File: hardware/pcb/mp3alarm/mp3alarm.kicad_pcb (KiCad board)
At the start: 2 copper layers, 67 x 54 mm, 30 parts, among them IC1 RDA5807FP, J0 debug, J1 AUDIO, J10 Conn_Coaxial, J2 SW0, J3 SW1, J4 SW2, J5 I2C, J6 TM1637, J7 microSD, J8 5V, J9 ANT, U1 UDA1334A_Breakout, U2 mini_esp32, Y1 Crystal

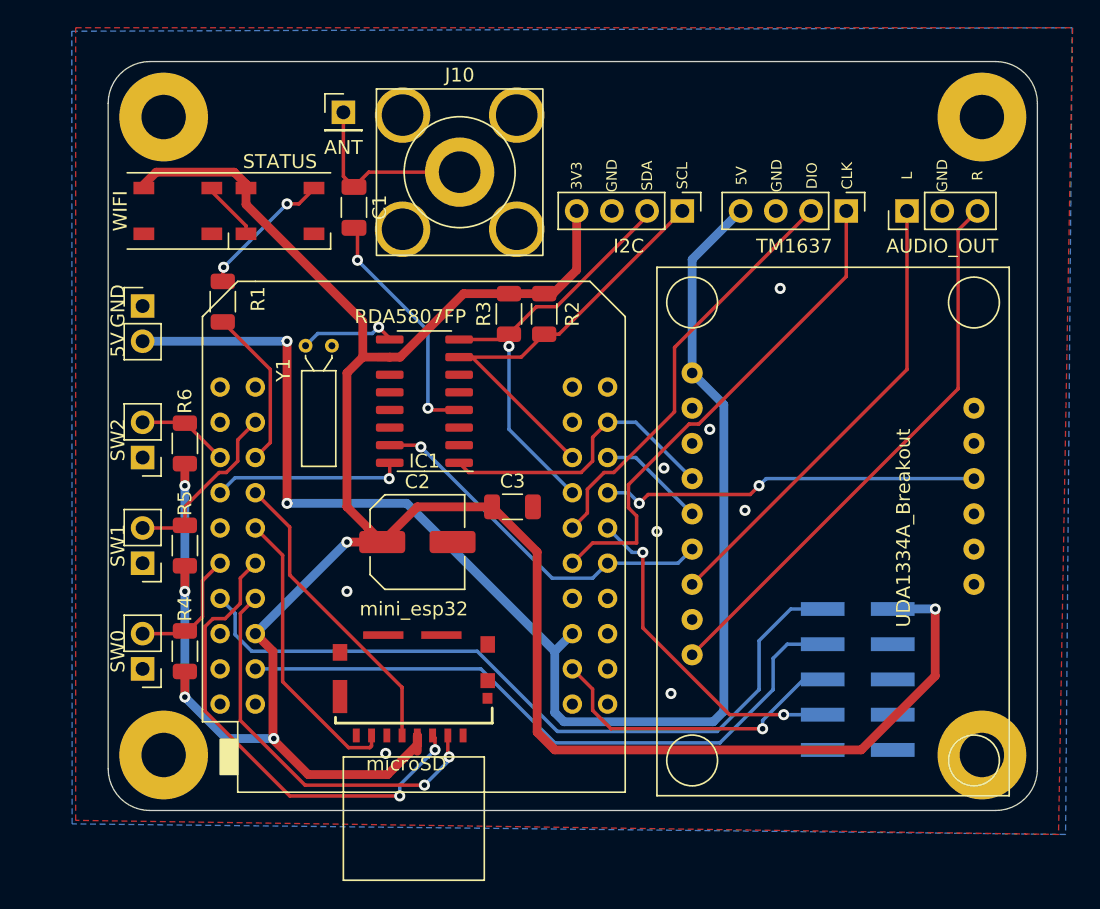
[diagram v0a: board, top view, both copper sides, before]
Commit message: * Latest PCB update for ESP32S3
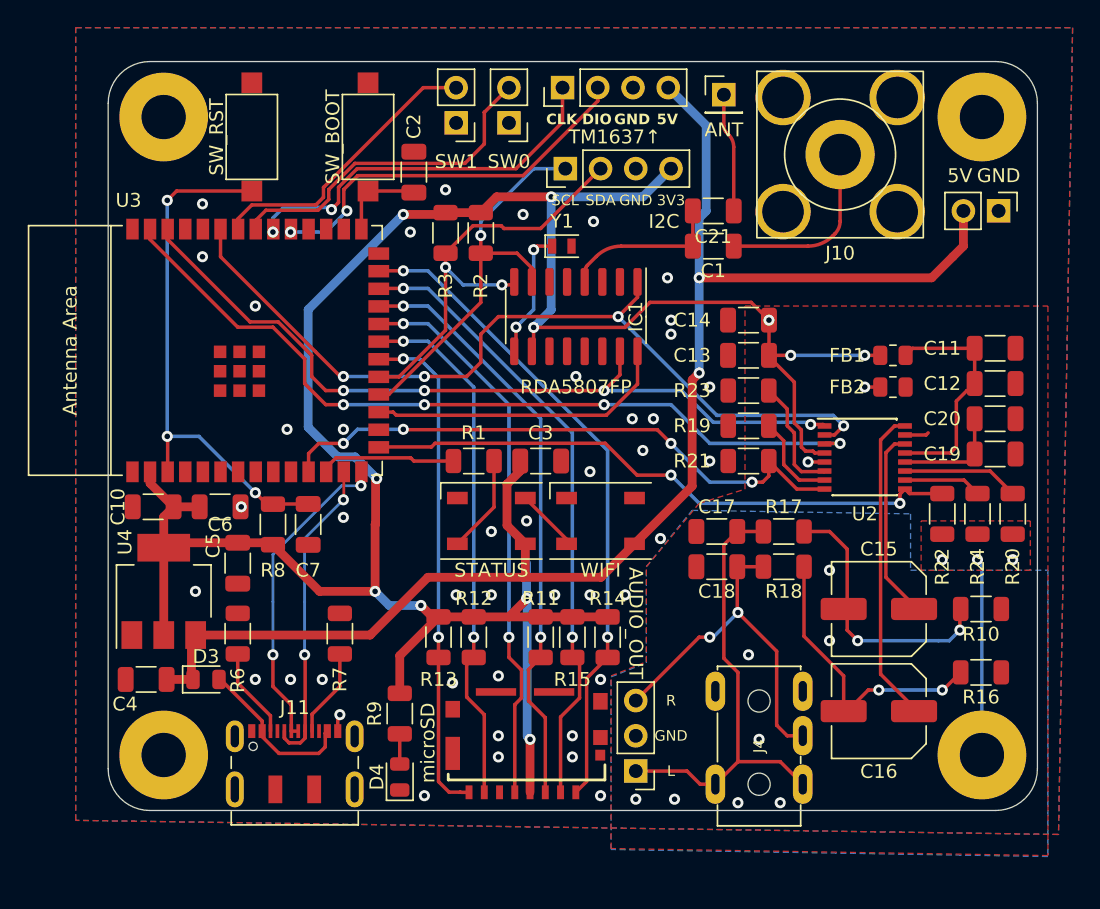
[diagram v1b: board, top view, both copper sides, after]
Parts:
- removed J0: debug, Connector_PinHeader_2.54mm:PinHeader_2x05_P2.54mm_Vertical_SMD
- removed R4, R5: 10k, Resistor_SMD:R_1206_3216Metric
- removed U1: UDA1334A_Breakout, UDA1334A:UDA1334A-breakout
- added C10: 0.1uF, Capacitor_SMD:C_1206_3216Metric, F.Cu at (47.2, 86.1)
- added C11: 0.1uF, Capacitor_SMD:C_1206_3216Metric, F.Cu at (108.0, 74.7)
- added C12: 10uF, Capacitor_SMD:C_1206_3216Metric, F.Cu at (108.0, 77.2)
- added C13: 0.1uF, Capacitor_SMD:C_1206_3216Metric, F.Cu at (90.2, 75.2)
- added C14: 10uF, Capacitor_SMD:C_1206_3216Metric, F.Cu at (90.2, 72.6)
- added C15: 47uF, Capacitor_SMD:C_Elec_6.3x5.4, F.Cu at (99.6, 93.5)
- added C16: 47uF, Capacitor_SMD:C_Elec_6.3x5.4, F.Cu at (99.6, 100.8)
- added C17: 0.01uF, Capacitor_SMD:C_1206_3216Metric, F.Cu at (87.9, 87.9)
- added C18: 0.01uF, Capacitor_SMD:C_1206_3216Metric, F.Cu at (87.9, 90.4)
- added C19: 0.1uF, Capacitor_SMD:C_1206_3216Metric, F.Cu at (108.0, 82.3)
- added C20: 10uF, Capacitor_SMD:C_1206_3216Metric, F.Cu at (108.0, 79.8)
- added C21: 1nF, Capacitor_SMD:C_1206_3216Metric, F.Cu at (87.6, 64.8)
- added C4: 10uF, Capacitor_SMD:C_1206_3216Metric, F.Cu at (46.7, 98.6)
- added C5: 10uF, Capacitor_SMD:C_1206_3216Metric, F.Cu at (53.3, 90.2)
- added C6: 22uF, Capacitor_SMD:C_1206_3216Metric, F.Cu at (52.1, 86.1)
- added C7: 1uF, Capacitor_SMD:C_1206_3216Metric, F.Cu at (58.4, 87.4)
- added D3: D_Schottky, Diode_SMD:D_0805_2012Metric, F.Cu at (51.1, 98.6)
- added D4: PWR, LED_SMD:LED_0805_2012Metric, F.Cu at (65.0, 105.6)
- added FB1: FerriteBead_Small, Resistor_SMD:R_0805_2012Metric, F.Cu at (100.6, 77.5)
- added FB2: FerriteBead_Small, Resistor_SMD:R_0805_2012Metric, F.Cu at (100.6, 75.2)
- added J11: USB_C_Receptacle_USB2.0, Connector_USB:USB_C_Receptacle_JAE_DX07S016JA1R1500, F.Cu at (57.5, 105.3)
- added R10: 220k, Resistor_SMD:R_1206_3216Metric, F.Cu at (106.9, 93.5)
- added R11: 10k, Resistor_SMD:R_1206_3216Metric, F.Cu at (75.2, 95.5)
- added R12: 10k, Resistor_SMD:R_1206_3216Metric, F.Cu at (70.4, 95.5)
- added R13: 10k, Resistor_SMD:R_1206_3216Metric, F.Cu at (67.8, 95.5)
- added R14: 10k, Resistor_SMD:R_1206_3216Metric, F.Cu at (80.0, 95.5)
- added R15: 10k, Resistor_SMD:R_1206_3216Metric, F.Cu at (77.5, 95.5)
- added R16: 220k, Resistor_SMD:R_1206_3216Metric, F.Cu at (106.9, 98.0)
- added R17: 100, Resistor_SMD:R_1206_3216Metric, F.Cu at (92.7, 87.9)
- added R18: 100, Resistor_SMD:R_1206_3216Metric, F.Cu at (92.7, 90.4)
- added R19: 10k, Resistor_SMD:R_1206_3216Metric, F.Cu at (90.2, 80.3)
- added R20: 10k, Resistor_SMD:R_1206_3216Metric, F.Cu at (109.2, 86.6)
- added R21: 10k, Resistor_SMD:R_1206_3216Metric, F.Cu at (90.2, 82.8)
- added R22: 10k, Resistor_SMD:R_1206_3216Metric, F.Cu at (104.1, 86.6)
- added R23: 10k, Resistor_SMD:R_1206_3216Metric, F.Cu at (90.2, 77.7)
- added R24: 10k, Resistor_SMD:R_1206_3216Metric, F.Cu at (106.7, 86.6)
- added R7: 5k1, Resistor_SMD:R_1206_3216Metric, F.Cu at (60.7, 95.2)
- added R8: 10k, Resistor_SMD:R_1206_3216Metric, F.Cu at (55.9, 87.4)
- added R9: 680, Resistor_SMD:R_1206_3216Metric, F.Cu at (65.0, 101.0)
- added SW1: SW_RST, Button_Switch_SMD:SW_SPST_CK_RS282G05A3, F.Cu at (54.4, 59.4)
- added SW2: SW_BOOT, Button_Switch_SMD:SW_SPST_CK_RS282G05A3, F.Cu at (62.7, 59.4)
- added U3: ESP32-S3-WROOM-1, PCM_Espressif:ESP32-S3-WROOM-1, F.Cu at (54.0, 74.8)
- added U4: AMS1117-3.3, Package_TO_SOT_SMD:SOT-223-3_TabPin2, F.Cu at (48.0, 92.2)
- C2: value 10uF -> 1uF; footprint Capacitor_SMD:C_Elec_6.3x5.4 -> Capacitor_SMD:C_1206_3216Metric
- C3: value 22nF -> 10uF
- J4: value SW2 -> AudioJack3; footprint Connector_PinHeader_2.54mm:PinHeader_1x02_P2.54mm_Vertical -> footprints:PJ-313
- R6: value 10k -> 5k1
- U2: value mini_esp32 -> UDA1334ATS; footprint pcb:ESP32_mini -> Package_SO:SSOP-16_4.4x5.2mm_P0.65mm
- Y1: footprint Crystal:Crystal_C26-LF_D2.1mm_L6.5mm_Horizontal -> Crystal:Crystal_SMD_2012-2Pin_2.0x1.2mm
- moved J8 62.1 mm to (108.2, 64.8), turned to -90 degrees
- moved J4 49.1 mm to (90.9, 103.4), turned to -90 degrees
- moved J2 47.4 mm to (72.9, 58.4)
- moved J1 44.9 mm to (82.0, 105.2), turned to 180 degrees
- moved J3 39.0 mm to (69.1, 58.4)
- moved D2 37.8 mm to (79.5, 87.1), turned to 180 degrees
- moved U2 33.1 mm to (98.6, 82.5)
- moved J10 27.5 mm to (96.8, 60.7)
- moved J9 27.5 mm to (88.4, 56.4)
- moved D1 27.1 mm to (71.6, 87.1), turned to 180 degrees
- moved C2 26.7 mm to (66.0, 62.0), turned to -90 degrees
- moved C1 26.1 mm to (87.6, 67.3), turned to 0 degrees
- moved J6 22.3 mm to (76.8, 55.9), turned to 90 degrees
- moved R1 21.4 mm to (70.4, 82.8), turned to 0 degrees
- moved Y1 19.8 mm to (76.7, 67.3)
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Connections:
- C1 pad 2: Net-(C1-Pad2) -> Net-(J10-In)
- C2 pad 1: VCC -> GND
- C2 pad 2: GND -> BOOT
- C3 pad 1: VCC -> GND
- C3 pad 2: GND -> +5V
- D1 pad 1: VCC -> +5V
- D2 pad 1: VCC -> +5V
- IC1 pad 4: Net-(C1-Pad2) -> ANT
- J1 pad 1: Net-(J1-Pad1) -> OUT_L
- J1 pad 2: GND -> GNDA
- J1 pad 3: Net-(J1-Pad3) -> OUT_R
- J10 pad 1: ANT -> Net-(J10-In)
- J6 pad 4: 5V -> +5V
- J7 pad 1: unconnected-(J7-Pad1) -> SD_D2
- J7 pad 2: SD_CD -> SD_D3
- J7 pad 7: SD_DATA0 -> SD_D0
- J7 pad 8: unconnected-(J7-Pad8) -> SD_D1
- J8 pad 2: 5V -> +5V
- J9 pad 1: ANT -> Net-(J9-Pin_1)
- R6 pad 1: VCC -> GND
- R6 pad 2: SW2 -> Net-(J11-CC1)
- U2 pad 1: GND -> I2S_BCLK
- U2 pad 10: SD_DATA0 -> Net-(U2-PLL0)
- U2 pad 11: SW0 -> Net-(U2-SFOR0)
- U2 pad 12: SD_CMD -> Net-(U2-Vref(DAC))
- U2 pad 13: TMS -> Net-(U2-VDDA)
- U2 pad 14: SD_CD -> Net-(U2-VOUTL)
- U2 pad 15: unconnected-(U2-Pad15) -> GNDA
- U2 pad 16: VCC -> Net-(U2-VOUTR)
- U2 pad 2: unconnected-(U2-Pad2) -> I2S_LRC
- U2 pad 3: unconnected-(U2-Pad3) -> I2S_DIN
- U2 pad 4: SW1 -> VCC
- U2 pad 5: SW2 -> GND
- U2 pad 6: STATUS_DATA -> Net-(U2-SYSCLK/PLL1)
- U2 pad 7: I2S_RADIO_DOUT -> Net-(U2-SFOR1)
- U2 pad 8: SD_CLK -> I2S_MUTE
- U2 pad 9: RDA_R -> I2S_DEEM
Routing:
- net +5V: track 0.00 -> 107.7 mm, vias 0 -> 2
- net 5V: track 103.3 -> 0.00 mm, vias 2 -> 0
- net TMS: track 54.0 -> 0.00 mm
- net I2S_DIN: track 7.78 -> 58.8 mm, vias 0 -> 4
- net SD_D2: track 0.00 -> 47.5 mm, vias 0 -> 2
- net TCK: track 47.4 -> 0.00 mm
- net SD_D3: track 0.00 -> 45.0 mm, vias 0 -> 2
- net I2S_DEEM: track 0.00 -> 43.5 mm, vias 0 -> 2
- net Net-(J1-Pad3): track 40.5 -> 0.00 mm
- net I2S_LRC: track 21.3 -> 61.5 mm, vias 0 -> 4
- net SD_D0: track 0.00 -> 38.2 mm, vias 0 -> 2
- net Net-(U3-EN): track 0.00 -> 38.1 mm, vias 0 -> 3
- net SD_D1: track 0.00 -> 36.5 mm, vias 0 -> 2
- net Net-(J1-Pad1): track 33.3 -> 0.00 mm
- net OUT_L: track 0.00 -> 33.2 mm
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- added copper zone on B.Cu, net GNDA
- added copper zone on F.Cu, net GNDA
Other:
- board text added: "ESP32 alarm clock v0.7"
- board text added: "TM1637↑"
- board text removed: "ESP32 alarm clock v0.5"
- board text removed: "NC"
- board text removed: "SW2"
- board text removed: "TCK"
- board text removed: "TDI"
- board text removed: "TDO"
- board text removed: "TM1637"
- board text removed: "TMS"
- board text removed: "VCC"
